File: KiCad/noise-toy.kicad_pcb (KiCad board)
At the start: 2 copper layers, 82.3 x 133.1 mm, 59 parts, among them J1 InputJack, J2 OutputJack, J3 Conn_02x20_PiZero, J4 Barrel_Jack_Switch, SW1 SWITCH_3PDT, SW2 SW_PUSH, SW3 SW_PUSH, SW4 SWITCH_INV, U1 MCP6002, U2 MCP3002

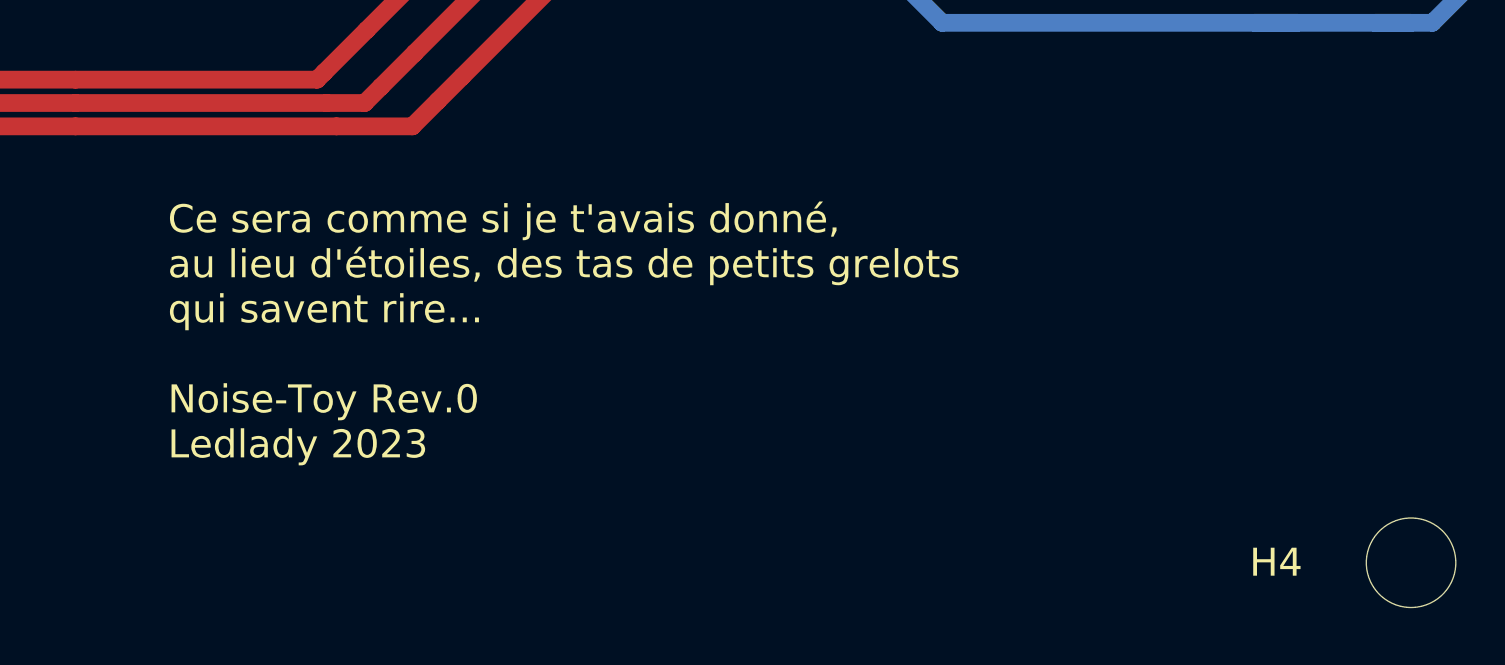
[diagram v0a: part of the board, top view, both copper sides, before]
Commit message: Added attribution to pcb
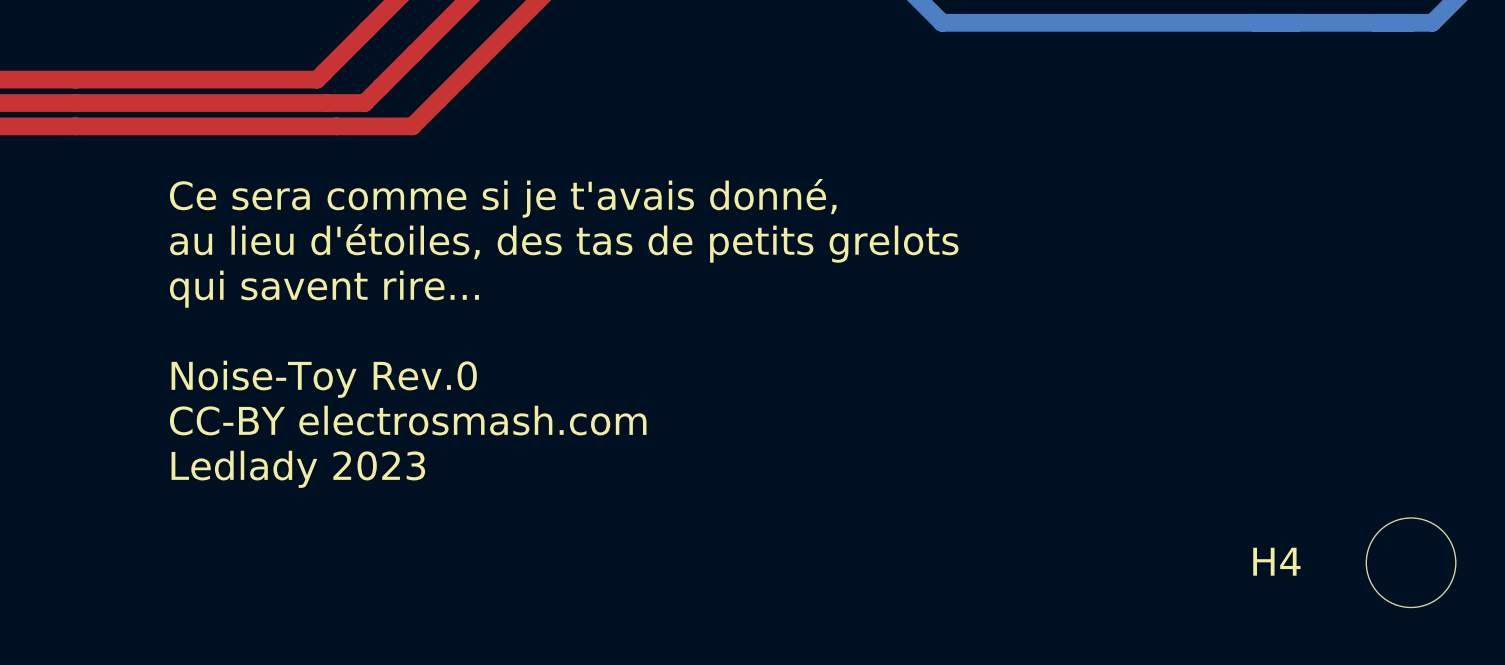
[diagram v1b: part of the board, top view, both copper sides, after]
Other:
- board text added: "Ce sera comme si je t'avais donné, au lieu d'étoiles, des tas de petits grelots qui savent rire... Noise-Toy Rev.0 CC-BY electrosmash.com Ledlady 2023"
- board text removed: "Ce sera comme si je t'avais donné, au lieu d'étoiles, des tas de petits grelots qui savent rire... Noise-Toy Rev.0 Ledlady 2023"
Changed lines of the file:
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@@
       (drillshape 0)
       (scaleselection 1)
-      (outputdirectory "gerber/")
+      (outputdirectory "../Production/GerberFiles/")
     )
   )
@@
   (gr_line (start 93.98 32.004) (end 176.276 32.004)
     (stroke (width 0.25) (type solid)) (layer "Edge.Cuts"))
-  (gr_text "Ce sera comme si je t'avais donné,\nau lieu d'étoiles, des tas de petits grelots\nqui savent rire... \n\nNoise-Toy Rev.0\nLedlady 2023" (at 125.476 150.495) (layer "F.SilkS")
+  (gr_text "Ce sera comme si je t'avais donné,\nau lieu d'étoiles, des tas de petits grelots\nqui savent rire... \n\nNoise-Toy Rev.0\nCC-BY electrosmash.com\nLedlady 2023" (at 125.476 150.495) (layer "F.SilkS")
     (effects (font (size 1 1) (thickness 0.2)) (justify left))
   )
